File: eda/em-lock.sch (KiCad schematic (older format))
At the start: 58 parts, among them P1 EXT_LED_CONN, P11 LEDA_CONN, P13 IN_LED_CONN, P14 LEDB_CONN, P15 LEDB_CONN, P2 RC522A, P3 RC522B, P4 BTN_OPEN, P5 BTN_CALL, P6 ESP8266_CONN, P7 LOCK_CONN, P8 LEDB_CONN, Q1 MMBT3906, Q2 MMBT3906, Q3 MMBT3906, Q4 MOSFET-NCHANNELSMD, U1 74LVC2G14

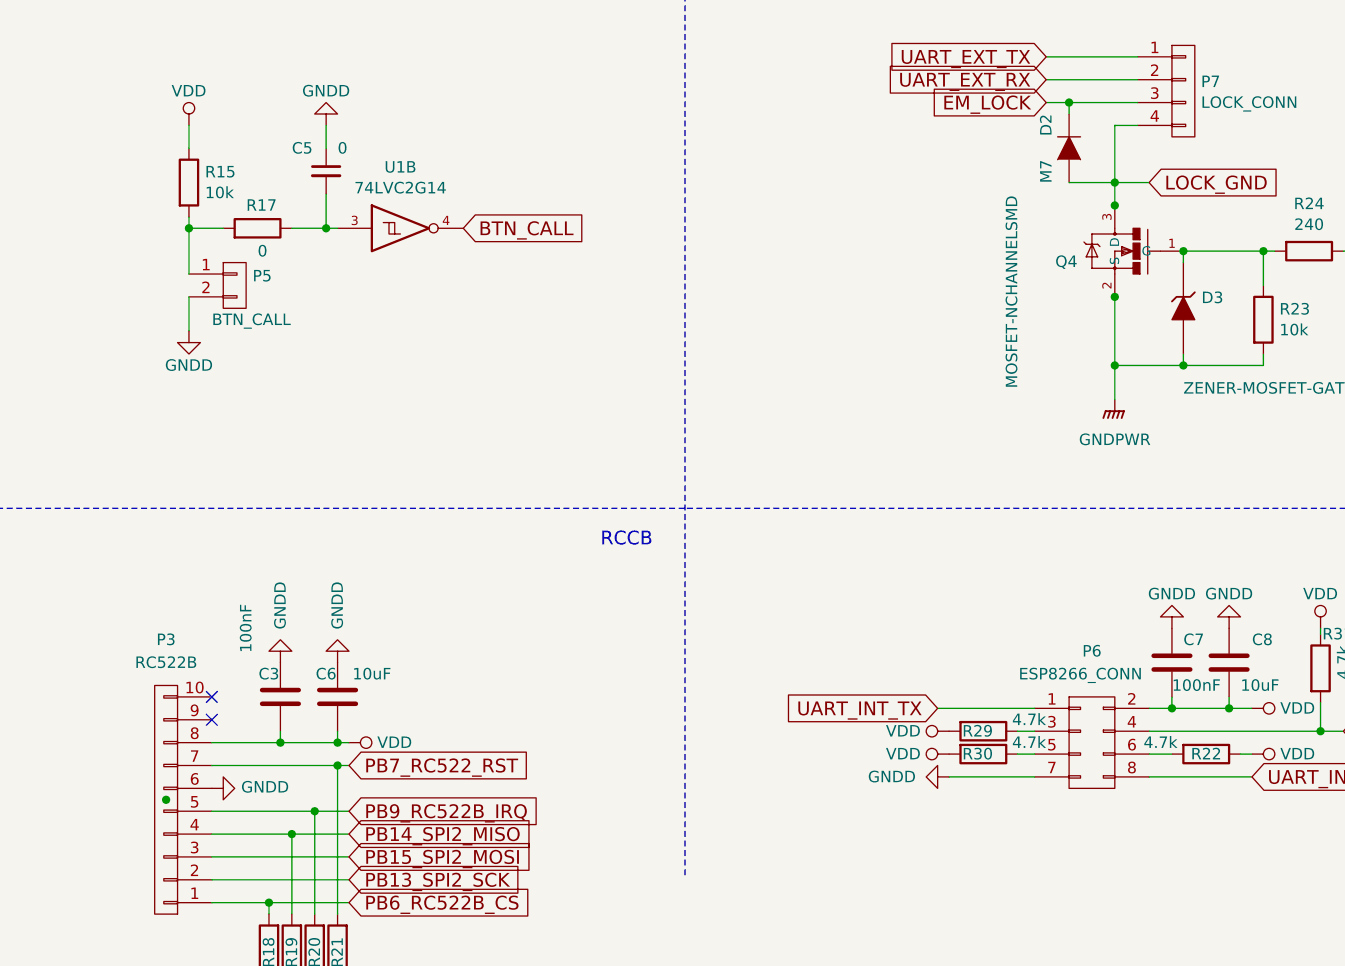
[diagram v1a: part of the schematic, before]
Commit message: Revert "Merge branch 'develop'"
This reverts commit ff1c94cd9af79a798b971b643cbdc9d823101f0c, reversing
changes made to 75416340a58c0ce3ae2d4917c1e5600380b4c8a3.
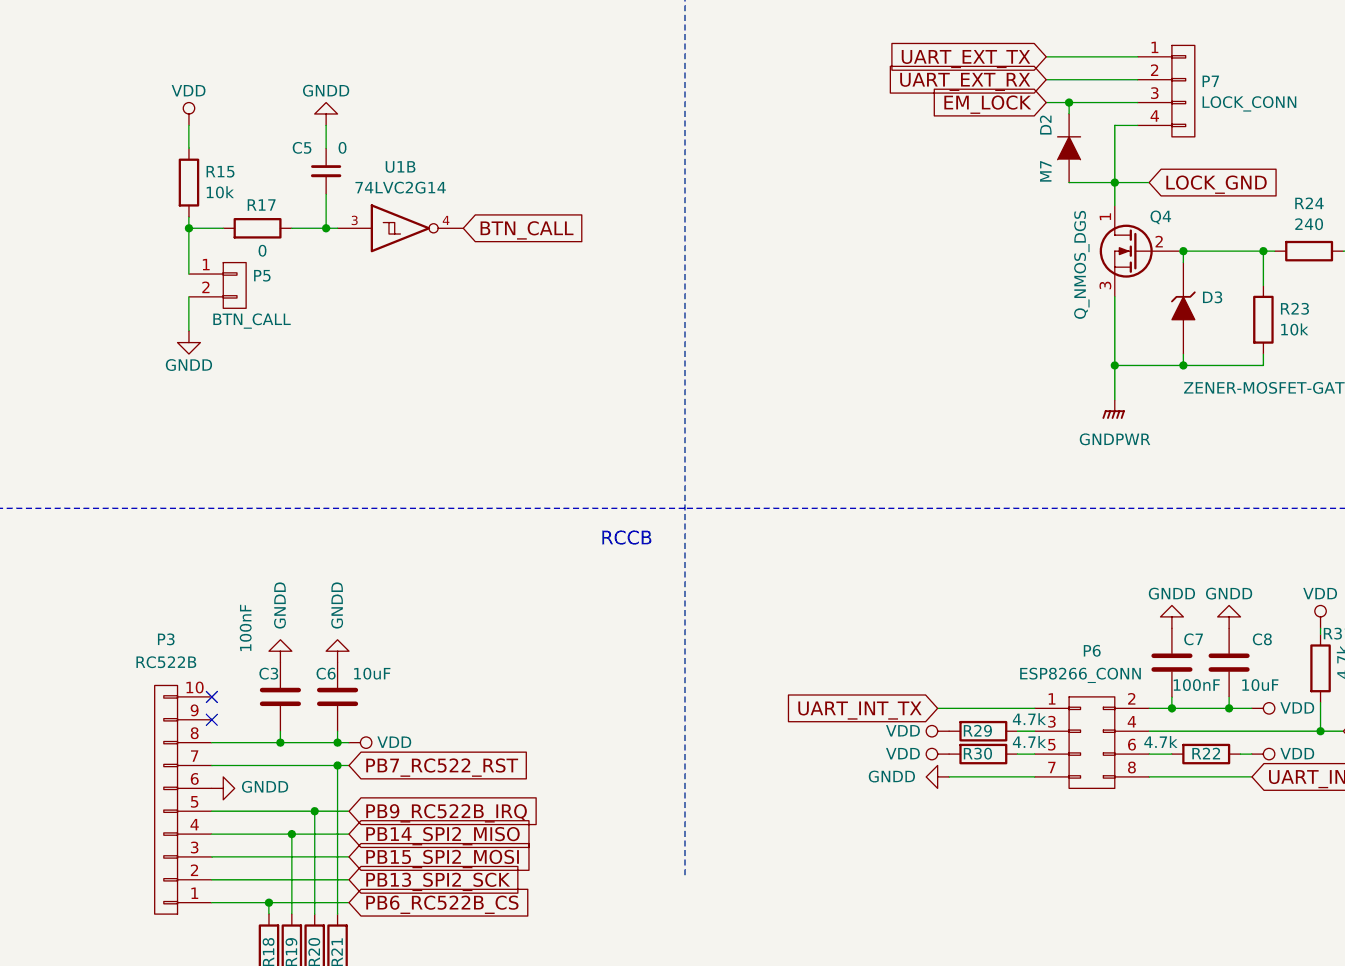
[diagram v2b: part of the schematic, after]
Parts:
- removed Q4: MOSFET-NCHANNELSMD, SparkFun-SOT23-3, symbol MOSFET-NCHANNELSMD
- added Q4: Q_NMOS_DGS, I20:SOT-23, symbol Q_NMOS_DGS
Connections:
- net GNDPWR: now also Q4.3 (S)
- net LOCK_GND: now also Q4.1 (D)
- net at D3.1 (K), R23.1, R24.2: now also Q4.2 (G)
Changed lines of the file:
@@
 EESchema Schematic File Version 2
+LIBS:em-lock-rescue
 LIBS:power
 LIBS:device
@@
 $EndComp
 $Comp
-L VDD #PWR01
+L VDD #PWR2
 U 1 1 57BF1F35
 P 1700 3000
-F 0 "#PWR01" H 1700 2850 50  0001 C CNN
+F 0 "#PWR2" H 1700 2850 50  0001 C CNN
 F 1 "VDD" H 1717 3173 50  0000 C CNN
 F 2 "" H 1700 3000 50  0000 C CNN
@@
 $EndComp
 $Comp
-L VDD #PWR02
+L VDD #PWR33
 U 1 1 57BFC190
 P 9450 5800
-F 0 "#PWR02" H 9450 5650 50  0001 C CNN
+F 0 "#PWR33" H 9450 5650 50  0001 C CNN
 F 1 "VDD" V 9450 6000 50  0000 C CNN
 F 2 "" H 9450 5800 50  0000 C CNN
@@
 	1    9100 5600
 	1    0    0    -1
+$EndComp
+$Comp
+L Q_NMOS_DGS Q4
+U 1 1 57BF2360
+P 8950 3800
+F 0 "Q4" H 8800 3950 50  0000 L CNN
+F 1 "Q_NMOS_DGS" V 9200 3500 50  0000 L CNN
+F 2 "I20:SOT-23" H 9150 3900 50  0001 C CNN
+F 3 "" H 8950 3800 50  0000 C CNN
+	1    8950 3800
+	-1   0    0    -1
 $EndComp
 $Comp
@@
 $EndComp
 $Comp
-L VDD #PWR03
+L VDD #PWR15
 U 1 1 57BFAAAC
 P 4800 3250
-F 0 "#PWR03" H 4800 3100 50  0001 C CNN
+F 0 "#PWR15" H 4800 3100 50  0001 C CNN
 F 1 "VDD" H 4800 3400 50  0000 C CNN
 F 2 "" H 4800 3250 50  0000 C CNN
@@
 $EndComp
 $Comp
-L GNDD #PWR04
+L GNDD #PWR10
 U 1 1 582803A4
 P 2800 950
-F 0 "#PWR04" H 2800 700 50  0001 C CNN
+F 0 "#PWR10" H 2800 700 50  0001 C CNN
 F 1 "GNDD" H 2800 800 50  0000 C CNN
 F 2 "" H 2800 950 50  0000 C CNN
@@
 $EndComp
 $Comp
-L VDD #PWR05
+L VDD #PWR9
 U 1 1 5829C375
 P 2250 6000
-F 0 "#PWR05" H 2250 5850 50  0001 C CNN
+F 0 "#PWR9" H 2250 5850 50  0001 C CNN
 F 1 "VDD" V 2250 6200 50  0000 C CNN
 F 2 "" H 2250 6000 50  0000 C CNN
@@
 $EndComp
 $Comp
-L GNDD #PWR06
+L GNDD #PWR1
 U 1 1 582EA563
 P 1650 6200
-F 0 "#PWR06" H 1650 5950 50  0001 C CNN
+F 0 "#PWR1" H 1650 5950 50  0001 C CNN
 F 1 "GNDD" V 1655 6072 50  0000 R CNN
 F 2 "" H 1650 6200 50  0000 C CNN
@@
 $EndComp
 $Comp
-L GNDD #PWR07
+L GNDD #PWR6
 U 1 1 582F6F93
 P 2100 7300
-F 0 "#PWR07" H 2100 7050 50  0001 C CNN
+F 0 "#PWR6" H 2100 7050 50  0001 C CNN
 F 1 "GNDD" V 2100 7050 50  0000 C CNN
 F 2 "" H 2100 7300 50  0000 C CNN
@@
 $EndComp
 $Comp
-L VDD #PWR08
+L VDD #PWR8
 U 1 1 582F7FA8
 P 2200 7300
-F 0 "#PWR08" H 2200 7150 50  0001 C CNN
+F 0 "#PWR8" H 2200 7150 50  0001 C CNN
 F 1 "VDD" V 2200 7500 50  0000 C CNN
 F 2 "" H 2200 7300 50  0000 C CNN
@@
 $EndComp
 $Comp
-L VDD #PWR09
+L VDD #PWR5
 U 1 1 582F87A4
 P 2000 7300
-F 0 "#PWR09" H 2000 7150 50  0001 C CNN
+F 0 "#PWR5" H 2000 7150 50  0001 C CNN
 F 1 "VDD" V 2000 7500 50  0000 C CNN
 F 2 "" H 2000 7300 50  0000 C CNN
@@
 $EndComp
 $Comp
-L VDD #PWR010
+L VDD #PWR3
 U 1 1 582F88B7
 P 1900 7300
-F 0 "#PWR010" H 1900 7150 50  0001 C CNN
+F 0 "#PWR3" H 1900 7150 50  0001 C CNN
 F 1 "VDD" V 1900 7500 50  0000 C CNN
 F 2 "" H 1900 7300 50  0000 C CNN
@@
 $EndComp
 $Comp
-L GNDD #PWR011
+L GNDD #PWR7
 U 1 1 582FC419
 P 2200 5650
-F 0 "#PWR011" H 2200 5400 50  0001 C CNN
+F 0 "#PWR7" H 2200 5400 50  0001 C CNN
 F 1 "GNDD" V 2200 5400 50  0000 C CNN
 F 2 "" H 2200 5650 50  0000 C CNN
@@
 $EndComp
 $Comp
-L GNDD #PWR012
+L GNDD #PWR4
 U 1 1 582FC718
 P 1950 5650
-F 0 "#PWR012" H 1950 5400 50  0001 C CNN
+F 0 "#PWR4" H 1950 5400 50  0001 C CNN
 F 1 "GNDD" V 1950 5400 50  0000 C CNN
 F 2 "" H 1950 5650 50  0000 C CNN
@@
 $EndComp
 $Comp
-L GNDD #PWR013
+L GNDD #PWR23
 U 1 1 58310A6A
 P 5400 3250
-F 0 "#PWR013" H 5400 3000 50  0001 C CNN
+F 0 "#PWR23" H 5400 3000 50  0001 C CNN
 F 1 "GNDD" H 5400 3100 50  0000 C CNN
 F 2 "" H 5400 3250 50  0000 C CNN
@@
 $EndComp
 $Comp
-L GNDD #PWR014
+L GNDD #PWR16
 U 1 1 58311616
 P 4800 4150
-F 0 "#PWR014" H 4800 3900 50  0001 C CNN
+F 0 "#PWR16" H 4800 3900 50  0001 C CNN
 F 1 "GNDD" H 4800 4000 50  0000 C CNN
 F 2 "" H 4800 4150 50  0000 C CNN
@@
 $EndComp
 $Comp
-L VDD #PWR015
+L VDD #PWR13
 U 1 1 5831B08E
 P 4800 1050
-F 0 "#PWR015" H 4800 900 50  0001 C CNN
+F 0 "#PWR13" H 4800 900 50  0001 C CNN
 F 1 "VDD" H 4800 1200 50  0000 C CNN
 F 2 "" H 4800 1050 50  0000 C CNN
@@
 $EndComp
 $Comp
-L GNDD #PWR016
+L GNDD #PWR22
 U 1 1 5831B0B3
 P 5400 1050
-F 0 "#PWR016" H 5400 800 50  0001 C CNN
+F 0 "#PWR22" H 5400 800 50  0001 C CNN
 F 1 "GNDD" H 5400 900 50  0000 C CNN
 F 2 "" H 5400 1050 50  0000 C CNN
@@
 $EndComp
 $Comp
-L GNDD #PWR017
+L GNDD #PWR14
 U 1 1 5831B0B9
 P 4800 1950
-F 0 "#PWR017" H 4800 1700 50  0001 C CNN
+F 0 "#PWR14" H 4800 1700 50  0001 C CNN
 F 1 "GNDD" H 4800 1800 50  0000 C CNN
 F 2 "" H 4800 1950 50  0000 C CNN
@@
 BTN_OPEN
 $Comp
-L VDD #PWR018
+L VDD #PWR26
 U 1 1 5835543A
 P 5500 5950
-F 0 "#PWR018" H 5500 5800 50  0001 C CNN
+F 0 "#PWR26" H 5500 5800 50  0001 C CNN
 F 1 "VDD" V 5500 6150 50  0000 C CNN
 F 2 "" H 5500 5950 50  0000 C CNN
@@
 $EndComp
 $Comp
-L GNDD #PWR019
+L GNDD #PWR17
 U 1 1 58355464
 P 4900 6150
-F 0 "#PWR019" H 4900 5900 50  0001 C CNN
+F 0 "#PWR17" H 4900 5900 50  0001 C CNN
 F 1 "GNDD" V 4905 6022 50  0000 R CNN
 F 2 "" H 4900 6150 50  0000 C CNN
@@
 $EndComp
 $Comp
-L GNDD #PWR020
+L GNDD #PWR21
 U 1 1 58355470
 P 5350 7250
-F 0 "#PWR020" H 5350 7000 50  0001 C CNN
+F 0 "#PWR21" H 5350 7000 50  0001 C CNN
 F 1 "GNDD" V 5350 7000 50  0000 C CNN
 F 2 "" H 5350 7250 50  0000 C CNN
@@
 $EndComp
 $Comp
-L VDD #PWR021
+L VDD #PWR25
 U 1 1 58355476
 P 5450 7250
-F 0 "#PWR021" H 5450 7100 50  0001 C CNN
+F 0 "#PWR25" H 5450 7100 50  0001 C CNN
 F 1 "VDD" V 5450 7450 50  0000 C CNN
 F 2 "" H 5450 7250 50  0000 C CNN
@@
 $EndComp
 $Comp
-L VDD #PWR022
+L VDD #PWR20
 U 1 1 5835547C
 P 5250 7250
-F 0 "#PWR022" H 5250 7100 50  0001 C CNN
+F 0 "#PWR20" H 5250 7100 50  0001 C CNN
 F 1 "VDD" V 5250 7450 50  0000 C CNN
 F 2 "" H 5250 7250 50  0000 C CNN
@@
 $EndComp
 $Comp
-L VDD #PWR023
+L VDD #PWR18
 U 1 1 58355482
 P 5150 7250
-F 0 "#PWR023" H 5150 7100 50  0001 C CNN
+F 0 "#PWR18" H 5150 7100 50  0001 C CNN
 F 1 "VDD" V 5150 7450 50  0000 C CNN
 F 2 "" H 5150 7250 50  0000 C CNN
@@
 $EndComp
 $Comp
-L GNDD #PWR024
+L GNDD #PWR24
 U 1 1 58355488
 P 5450 5600
-F 0 "#PWR024" H 5450 5350 50  0001 C CNN
+F 0 "#PWR24" H 5450 5350 50  0001 C CNN
 F 1 "GNDD" V 5450 5350 50  0000 C CNN
 F 2 "" H 5450 5600 50  0000 C CNN
@@
 $EndComp
 $Comp
-L GNDD #PWR025
+L GNDD #PWR19
 U 1 1 5835548E
 P 5200 5600
-F 0 "#PWR025" H 5200 5350 50  0001 C CNN
+F 0 "#PWR19" H 5200 5350 50  0001 C CNN
 F 1 "GNDD" V 5200 5350 50  0000 C CNN
 F 2 "" H 5200 5600 50  0000 C CNN
@@
 RCCA
 $Comp
-L GNDD #PWR026
+L GNDD #PWR32
 U 1 1 583814D2
 P 9350 5450
-F 0 "#PWR026" H 9350 5200 50  0001 C CNN
+F 0 "#PWR32" H 9350 5200 50  0001 C CNN
 F 1 "GNDD" H 9350 5300 50  0000 C CNN
 F 2 "" H 9350 5450 50  0000 C CNN
@@
 $EndComp
 $Comp
-L GNDD #PWR027
+L GNDD #PWR29
 U 1 1 58381774
 P 8125 6100
-F 0 "#PWR027" H 8125 5850 50  0001 C CNN
+F 0 "#PWR29" H 8125 5850 50  0001 C CNN
 F 1 "GNDD" V 8125 5850 50  0000 C CNN
 F 2 "" H 8125 6100 50  0000 C CNN
@@
 $EndComp
 $Comp
-L GNDD #PWR028
+L GNDD #PWR31
 U 1 1 583AE5EE
 P 9100 5450
-F 0 "#PWR028" H 9100 5200 50  0001 C CNN
+F 0 "#PWR31" H 9100 5200 50  0001 C CNN
 F 1 "GNDD" H 9100 5300 50  0000 C CNN
 F 2 "" H 9100 5450 50  0000 C CNN
@@
 $EndComp
 $Comp
-L VDD #PWR029
+L VDD #PWR34
 U 1 1 583B6020
 P 9450 6000
-F 0 "#PWR029" H 9450 5850 50  0001 C CNN
+F 0 "#PWR34" H 9450 5850 50  0001 C CNN
 F 1 "VDD" V 9450 6200 50  0000 C CNN
 F 2 "" H 9450 6000 50  0000 C CNN
@@
 $EndComp
 $Comp
-L VDD #PWR030
+L VDD #PWR11
 U 1 1 58223ACA
 P 3150 1050
-F 0 "#PWR030" H 3150 900 50  0001 C CNN
+F 0 "#PWR11" H 3150 900 50  0001 C CNN
 F 1 "VDD" V 3150 1250 50  0000 C CNN
 F 2 "" H 3150 1050 50  0000 C CNN
@@
 $EndComp
 $Comp
-L VDD #PWR031
+L VDD #PWR12
 U 1 1 582264A1
 P 3150 1250
-F 0 "#PWR031" H 3150 1100 50  0001 C CNN
+F 0 "#PWR12" H 3150 1100 50  0001 C CNN
 F 1 "VDD" V 3150 1450 50  0000 C CNN
 F 2 "" H 3150 1250 50  0000 C CNN
@@
 EM_LOCK
 $Comp
-L GNDPWR #PWR032
+L GNDPWR #PWR30
 U 1 1 58586DF6
 P 8850 4450
-F 0 "#PWR032" H 8850 4250 50  0001 C CNN
+F 0 "#PWR30" H 8850 4250 50  0001 C CNN
 F 1 "GNDPWR" H 8850 4275 50  0000 C CNN
 F 2 "" H 8850 4400 50  0000 C CNN
@@
 $EndComp
 $Comp
-L VDD #PWR033
+L VDD #PWR28
 U 1 1 58718815
 P 8125 6000
-F 0 "#PWR033" H 8125 5850 50  0001 C CNN
+F 0 "#PWR28" H 8125 5850 50  0001 C CNN
 F 1 "VDD" V 8125 6200 50  0000 C CNN
 F 2 "" H 8125 6000 50  0000 C CNN
@@
 $EndComp
 $Comp
-L VDD #PWR034
+L VDD #PWR27
 U 1 1 5871B4C1
 P 8125 5900
-F 0 "#PWR034" H 8125 5750 50  0001 C CNN
+F 0 "#PWR27" H 8125 5750 50  0001 C CNN
 F 1 "VDD" V 8125 6100 50  0000 C CNN
 F 2 "" H 8125 5900 50  0000 C CNN
@@
 $EndComp
 $Comp
-L VDD #PWR035
+L VDD #PWR35
 U 1 1 58729F36
 P 9750 5450
-F 0 "#PWR035" H 9750 5300 50  0001 C CNN
+F 0 "#PWR35" H 9750 5300 50  0001 C CNN
 F 1 "VDD" H 9750 5600 50  0000 C CNN
 F 2 "" H 9750 5450 50  0000 C CNN
@@
 Wire Wire Line
 	9500 4300 9500 4250
+Connection ~ 8850 4300
 Wire Wire Line
 	8850 4300 9500 4300
+Connection ~ 9150 3800
 Wire Wire Line
 	9150 3850 9150 3800
@@
 Wire Wire Line
 	9000 5900 9850 5900
-$Comp
-L MOSFET-NCHANNELSMD Q4
-U 1 1 58A34D60
-P 8850 3800
-F 0 "Q4" H 9013 3754 50  0000 L CNN
-F 1 "MOSFET-NCHANNELSMD" V 9300 3200 50  0000 L CNN
-F 2 "SparkFun-SOT23-3" H 9400 3800 50  0001 C CNN
-F 3 "" H 8850 3800 60  0001 C CNN
-	1    8850 3800
-	-1   0    0    -1
-$EndComp
-Connection ~ 8850 4300
-Connection ~ 9150 3800
-Connection ~ 4700 6200
-Connection ~ 8850 3600
-Connection ~ 8850 4000
 $EndSCHEMATC
